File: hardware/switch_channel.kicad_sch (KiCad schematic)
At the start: 9 parts, among them J6 Screw_Terminal_01x02, Q10 BUZ11, Q9 BC847

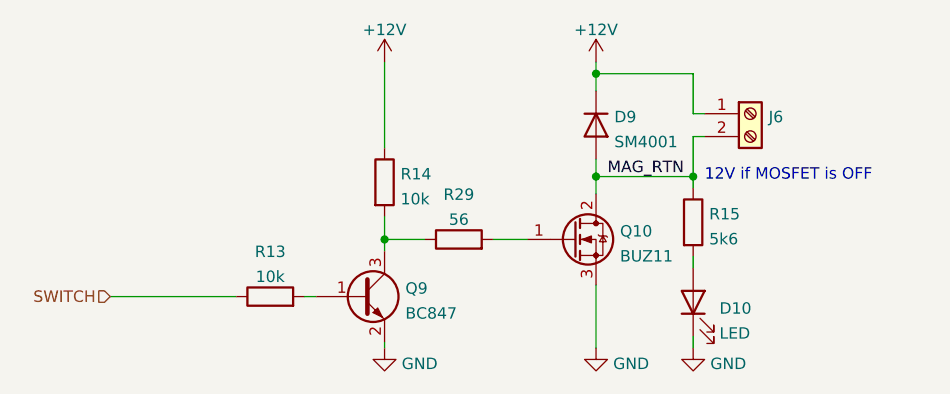
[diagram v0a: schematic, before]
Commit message: first iteration of layout almost done
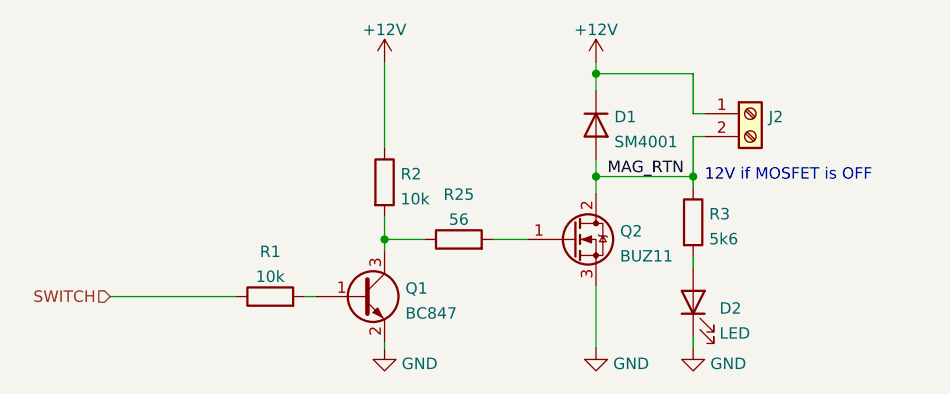
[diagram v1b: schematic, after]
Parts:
- renumbered D9 to D1, D10 to D2, J6 to J2, Q9 to Q1, Q10 to Q2, R13 to R1, R14 to R2, R29 to R25, R15 to R3
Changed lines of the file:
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@@
   (symbol (lib_id "Diode:SM4001") (at 136.525 73.66 270)
     (in_bom yes) (on_board yes) (fields_autoplaced)
-    (property "Reference" "D9" (id 0) (at 138.557 72.7515 90)
+    (property "Reference" "D1" (id 0) (at 138.557 72.7515 90)
       (effects (font (size 1.27 1.27)) (justify left))
     )
@@
   (symbol (lib_id "power:+12V") (at 113.03 66.675 0)
     (in_bom yes) (on_board yes) (fields_autoplaced)
-    (property "Reference" "#PWR024" (id 0) (at 113.03 70.485 0)
+    (property "Reference" "#PWR04" (id 0) (at 113.03 70.485 0)
       (effects (font (size 1.27 1.27)) hide)
     )
@@
   (symbol (lib_id "power:GND") (at 136.525 98.425 0) (mirror y)
     (in_bom yes) (on_board yes) (fields_autoplaced)
-    (property "Reference" "#PWR027" (id 0) (at 136.525 104.775 0)
+    (property "Reference" "#PWR07" (id 0) (at 136.525 104.775 0)
       (effects (font (size 1.27 1.27)) hide)
     )
@@
   (symbol (lib_id "Device:R") (at 113.03 80.01 0)
     (in_bom yes) (on_board yes)
-    (property "Reference" "R14" (id 0) (at 114.808 79.1015 0)
+    (property "Reference" "R2" (id 0) (at 114.808 79.1015 0)
       (effects (font (size 1.27 1.27)) (justify left))
     )
@@
   (symbol (lib_id "power:GND") (at 147.32 98.425 0) (mirror y)
     (in_bom yes) (on_board yes) (fields_autoplaced)
-    (property "Reference" "#PWR028" (id 0) (at 147.32 104.775 0)
+    (property "Reference" "#PWR08" (id 0) (at 147.32 104.775 0)
       (effects (font (size 1.27 1.27)) hide)
     )
@@
   (symbol (lib_id "power:GND") (at 113.03 98.425 0) (mirror y)
     (in_bom yes) (on_board yes) (fields_autoplaced)
-    (property "Reference" "#PWR025" (id 0) (at 113.03 104.775 0)
+    (property "Reference" "#PWR05" (id 0) (at 113.03 104.775 0)
       (effects (font (size 1.27 1.27)) hide)
     )
@@
   (symbol (lib_id "Transistor_FET:BUZ11") (at 133.985 86.36 0)
     (in_bom yes) (on_board yes) (fields_autoplaced)
-    (property "Reference" "Q10" (id 0) (at 139.192 85.4515 0)
+    (property "Reference" "Q2" (id 0) (at 139.192 85.4515 0)
       (effects (font (size 1.27 1.27)) (justify left))
     )
@@
   (symbol (lib_id "Device:R") (at 147.32 84.455 0)
     (in_bom yes) (on_board yes) (fields_autoplaced)
-    (property "Reference" "R15" (id 0) (at 149.098 83.5465 0)
+    (property "Reference" "R3" (id 0) (at 149.098 83.5465 0)
       (effects (font (size 1.27 1.27)) (justify left))
     )
@@
   (symbol (lib_id "Transistor_BJT:BC847") (at 110.49 92.71 0)
     (in_bom yes) (on_board yes) (fields_autoplaced)
-    (property "Reference" "Q9" (id 0) (at 115.3414 91.8015 0)
+    (property "Reference" "Q1" (id 0) (at 115.3414 91.8015 0)
       (effects (font (size 1.27 1.27)) (justify left))
     )
@@
   (symbol (lib_id "Device:R") (at 121.285 86.36 90)
     (in_bom yes) (on_board yes) (fields_autoplaced)
-    (property "Reference" "R29" (id 0) (at 121.285 81.3775 90))
+    (property "Reference" "R25" (id 0) (at 121.285 81.3775 90))
     (property "Value" "56" (id 1) (at 121.285 84.1526 90))
     (property "Footprint" "Resistor_SMD:R_0603_1608Metric" (id 2) (at 121.285 88.138 90)
@@
   (symbol (lib_id "Device:R") (at 100.33 92.71 90)
     (in_bom yes) (on_board yes) (fields_autoplaced)
-    (property "Reference" "R13" (id 0) (at 100.33 87.7275 90))
+    (property "Reference" "R1" (id 0) (at 100.33 87.7275 90))
     (property "Value" "10k" (id 1) (at 100.33 90.5026 90))
     (property "Footprint" "Resistor_SMD:R_0603_1608Metric" (id 2) (at 100.33 94.488 90)
@@
   (symbol (lib_id "power:+12V") (at 136.525 66.675 0)
     (in_bom yes) (on_board yes) (fields_autoplaced)
-    (property "Reference" "#PWR026" (id 0) (at 136.525 70.485 0)
+    (property "Reference" "#PWR06" (id 0) (at 136.525 70.485 0)
       (effects (font (size 1.27 1.27)) hide)
     )
@@
   (symbol (lib_id "Connector:Screw_Terminal_01x02") (at 153.67 72.39 0)
     (in_bom yes) (on_board yes) (fields_autoplaced)
-    (property "Reference" "J6" (id 0) (at 155.702 72.7515 0)
+    (property "Reference" "J2" (id 0) (at 155.702 72.7515 0)
       (effects (font (size 1.27 1.27)) (justify left))
     )
@@
   (symbol (lib_id "Device:LED") (at 147.32 93.345 90)
     (in_bom yes) (on_board yes) (fields_autoplaced)
-    (property "Reference" "D10" (id 0) (at 150.241 94.024 90)
-      (effects (font (size 1.27 1.27)) (justify right))
-    )
+    (property "Reference" "D2" (id 0) (at 150.241 94.024 90)
+      (effects (font (size 1.27 1.27)) (justify right))
+    )

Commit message: added 7805 as voltage regulator
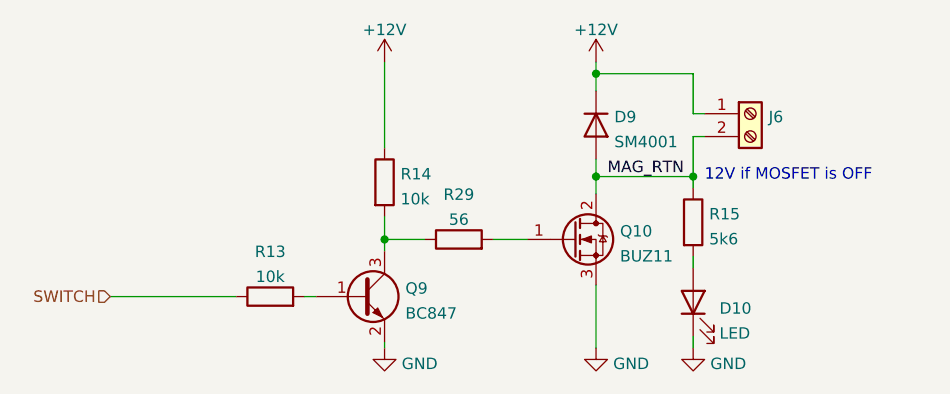
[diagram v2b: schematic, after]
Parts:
- renumbered D2 to D10, D1 to D9, J2 to J6, Q2 to Q10, Q1 to Q9, R1 to R13, R2 to R14, R3 to R15, R25 to R29
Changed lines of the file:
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@@
   (symbol (lib_id "Diode:SM4001") (at 136.525 73.66 270)
     (in_bom yes) (on_board yes) (fields_autoplaced)
-    (property "Reference" "D1" (id 0) (at 138.557 72.7515 90)
+    (property "Reference" "D9" (id 0) (at 138.557 72.7515 90)
       (effects (font (size 1.27 1.27)) (justify left))
     )
@@
   (symbol (lib_id "power:+12V") (at 113.03 66.675 0)
     (in_bom yes) (on_board yes) (fields_autoplaced)
-    (property "Reference" "#PWR04" (id 0) (at 113.03 70.485 0)
+    (property "Reference" "#PWR024" (id 0) (at 113.03 70.485 0)
       (effects (font (size 1.27 1.27)) hide)
     )
@@
   (symbol (lib_id "power:GND") (at 136.525 98.425 0) (mirror y)
     (in_bom yes) (on_board yes) (fields_autoplaced)
-    (property "Reference" "#PWR07" (id 0) (at 136.525 104.775 0)
+    (property "Reference" "#PWR027" (id 0) (at 136.525 104.775 0)
       (effects (font (size 1.27 1.27)) hide)
     )
@@
   (symbol (lib_id "Device:R") (at 113.03 80.01 0)
     (in_bom yes) (on_board yes)
-    (property "Reference" "R2" (id 0) (at 114.808 79.1015 0)
+    (property "Reference" "R14" (id 0) (at 114.808 79.1015 0)
       (effects (font (size 1.27 1.27)) (justify left))
     )
@@
   (symbol (lib_id "power:GND") (at 147.32 98.425 0) (mirror y)
     (in_bom yes) (on_board yes) (fields_autoplaced)
-    (property "Reference" "#PWR08" (id 0) (at 147.32 104.775 0)
+    (property "Reference" "#PWR028" (id 0) (at 147.32 104.775 0)
       (effects (font (size 1.27 1.27)) hide)
     )
@@
   (symbol (lib_id "power:GND") (at 113.03 98.425 0) (mirror y)
     (in_bom yes) (on_board yes) (fields_autoplaced)
-    (property "Reference" "#PWR05" (id 0) (at 113.03 104.775 0)
+    (property "Reference" "#PWR025" (id 0) (at 113.03 104.775 0)
       (effects (font (size 1.27 1.27)) hide)
     )
@@
   (symbol (lib_id "Transistor_FET:BUZ11") (at 133.985 86.36 0)
     (in_bom yes) (on_board yes) (fields_autoplaced)
-    (property "Reference" "Q2" (id 0) (at 139.192 85.4515 0)
+    (property "Reference" "Q10" (id 0) (at 139.192 85.4515 0)
       (effects (font (size 1.27 1.27)) (justify left))
     )
@@
   (symbol (lib_id "Device:R") (at 147.32 84.455 0)
     (in_bom yes) (on_board yes) (fields_autoplaced)
-    (property "Reference" "R3" (id 0) (at 149.098 83.5465 0)
+    (property "Reference" "R15" (id 0) (at 149.098 83.5465 0)
       (effects (font (size 1.27 1.27)) (justify left))
     )
@@
   (symbol (lib_id "Transistor_BJT:BC847") (at 110.49 92.71 0)
     (in_bom yes) (on_board yes) (fields_autoplaced)
-    (property "Reference" "Q1" (id 0) (at 115.3414 91.8015 0)
+    (property "Reference" "Q9" (id 0) (at 115.3414 91.8015 0)
       (effects (font (size 1.27 1.27)) (justify left))
     )
@@
   (symbol (lib_id "Device:R") (at 121.285 86.36 90)
     (in_bom yes) (on_board yes) (fields_autoplaced)
-    (property "Reference" "R25" (id 0) (at 121.285 81.3775 90))
+    (property "Reference" "R29" (id 0) (at 121.285 81.3775 90))
     (property "Value" "56" (id 1) (at 121.285 84.1526 90))
     (property "Footprint" "Resistor_SMD:R_0603_1608Metric" (id 2) (at 121.285 88.138 90)
@@
   (symbol (lib_id "Device:R") (at 100.33 92.71 90)
     (in_bom yes) (on_board yes) (fields_autoplaced)
-    (property "Reference" "R1" (id 0) (at 100.33 87.7275 90))
+    (property "Reference" "R13" (id 0) (at 100.33 87.7275 90))
     (property "Value" "10k" (id 1) (at 100.33 90.5026 90))
     (property "Footprint" "Resistor_SMD:R_0603_1608Metric" (id 2) (at 100.33 94.488 90)
@@
   (symbol (lib_id "power:+12V") (at 136.525 66.675 0)
     (in_bom yes) (on_board yes) (fields_autoplaced)
-    (property "Reference" "#PWR06" (id 0) (at 136.525 70.485 0)
+    (property "Reference" "#PWR026" (id 0) (at 136.525 70.485 0)
       (effects (font (size 1.27 1.27)) hide)
     )
@@
   (symbol (lib_id "Connector:Screw_Terminal_01x02") (at 153.67 72.39 0)
     (in_bom yes) (on_board yes) (fields_autoplaced)
-    (property "Reference" "J2" (id 0) (at 155.702 72.7515 0)
+    (property "Reference" "J6" (id 0) (at 155.702 72.7515 0)
       (effects (font (size 1.27 1.27)) (justify left))
     )
@@
   (symbol (lib_id "Device:LED") (at 147.32 93.345 90)
     (in_bom yes) (on_board yes) (fields_autoplaced)
-    (property "Reference" "D2" (id 0) (at 150.241 94.024 90)
-      (effects (font (size 1.27 1.27)) (justify right))
-    )
+    (property "Reference" "D10" (id 0) (at 150.241 94.024 90)
+      (effects (font (size 1.27 1.27)) (justify right))
+    )
